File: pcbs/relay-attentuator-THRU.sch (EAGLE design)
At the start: 25 parts, among them IC1 ULN2803, IC2 MCP23S08, K1 IM23TS, K2 IM43TS, K3 IM43TS, K4 IM43TS, X1 22-23-2051

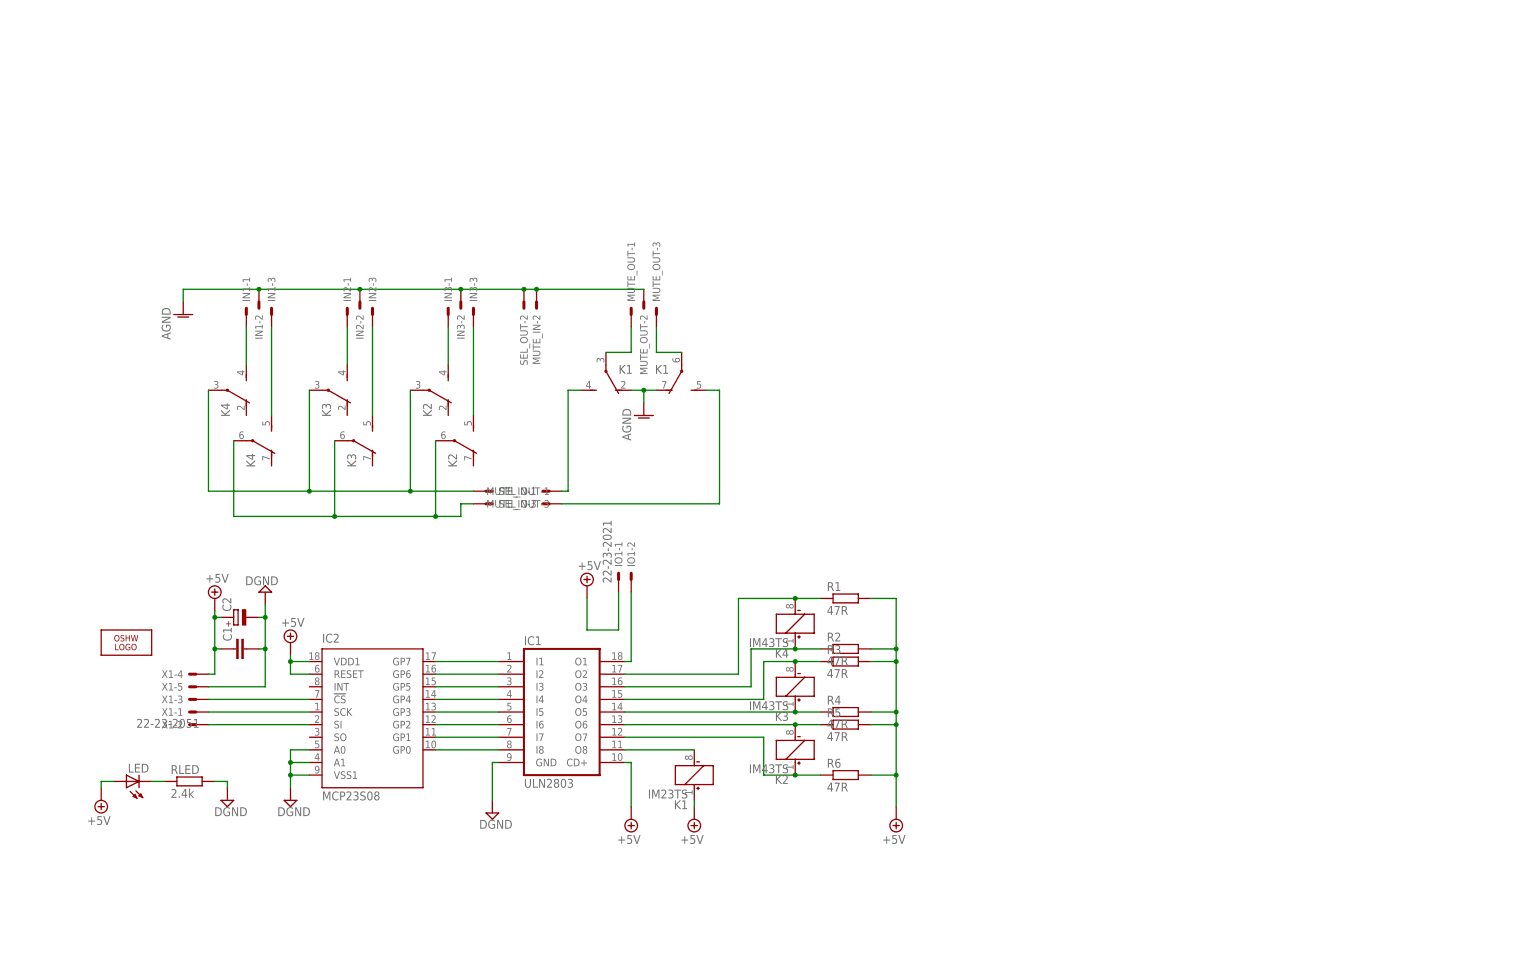
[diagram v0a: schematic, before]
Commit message: new designs
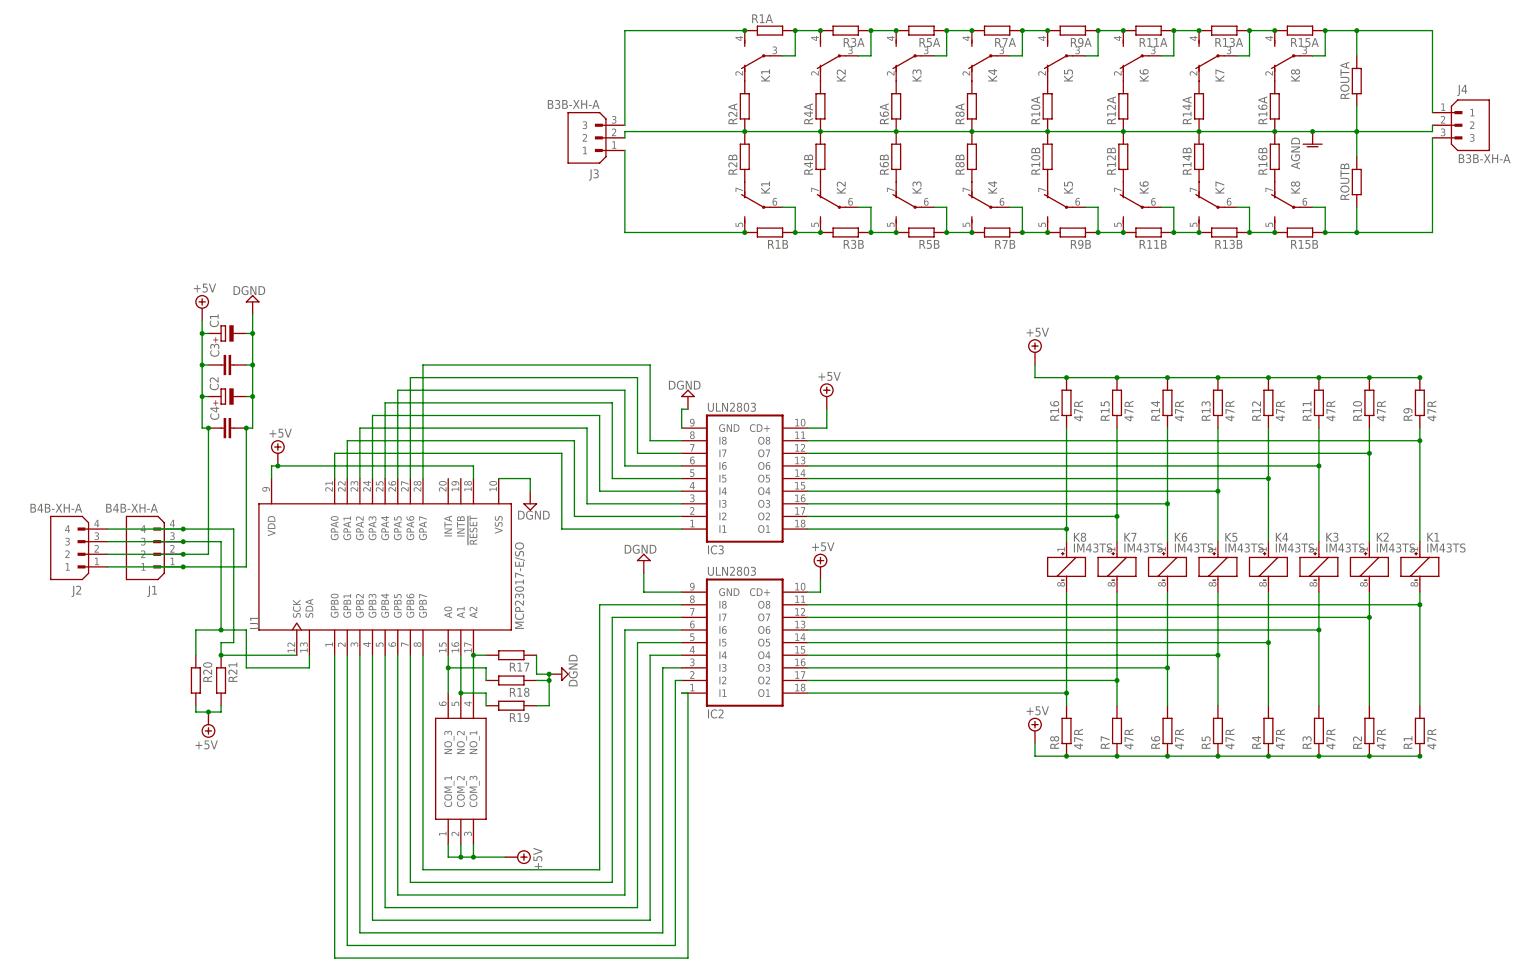
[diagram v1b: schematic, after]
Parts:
- removed IC1: ULN2803, uln-udn-mine:ULN2803ADW
- removed IN1, IN2, IN3, MUTE_IN, MUTE_OUT, SEL_OUT: 22-23-2031, con-molex:22-23-2031
- removed IO1: 22-23-2021, con-molex:22-23-2021
- removed LED: (no value), led:LEDCHIPLED_1206
- removed LOGO1: OSHW_LOGO_FILLX0200-NT, ohw-logo:OSHW_LOGO_FILLX0200-NT
- removed RLED: 2.4k, rcl:R-EU_R1206
- removed X1: 22-23-2051, con-molex:22-23-2051
- added C3, C4: (no value), rcl:C-EUC1206
- added IC3: ULN2803, uln-udn-mine:ULN2803ADW
- added J1, J2: B4B-XH-A, B4B-XH-A:B4B-XH-A
- added J3, J4: B3B-XH-A, B3B-XH-A:B3B-XH-A
- added K5, K6, K7, K8: IM43TS, relay-te:IM43TS
- added R10, R11, R12, R13, R14, R15, R16, R17, R18, R19, R20, R21, R7, R8, R9: 47R, rcl:R-EU_R1206
- added R10A, R10B, R11A, R11B, R12A, R12B, R13A, R13B, R14A, R14B, R15A, R15B, R16A, R16B, R1A, R1B, R2A, R2B, R3A, R3B, R4A, R4B, R5A, R5B, R6A, R6B, R7A, R7B, R8A, R8B, R9A, R9B, ROUTA, ROUTB: (no value), rcl:R-EU_0207/10
- added S1: 2454982-2, 2454982-2:2454982-2
- added U1: MCP23017-E/SO, MCP23017-E_SO:MCP23017-E/SO
- C1: device rcl:C-EUC1206 -> rcl:CPOL-EUE3.5-8
- C2: device rcl:CPOL-EUC -> rcl:CPOL-EUE3.5-8
- IC2: value MCP23S08 -> ULN2803; device microchip-mine:MCP23S08-E/SO -> uln-udn-mine:ULN2803ADW
- K1: value IM23TS -> IM43TS; device relay-te:IM23TS -> relay-te:IM43TS
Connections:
- removed net CS: IC2.!CS, X1-3.S
- removed net INL: K22.P, K32.P, K42.P, SEL_OUT-1.S
- removed net INR: K23.P, K33.P, K43.P, SEL_OUT-3.S
- removed net N$67: LED.C, RLED.1
- removed net OUTL: K12.S, MUTE_IN-1.S
- removed net OUTR: K13.S, MUTE_IN-3.S
- removed net SCK: IC2.SCK, X1-1.S
- removed net SI: IC2.SI, X1-2.S
- new net ATT_INR: J3.1, K13.S, R1B.2
- new net N$114: K32.P, K42.S, R5A.1, R7A.2
- new net N$115: K42.P, K52.S, R7A.1, R9A.2
- new net N$116: K52.P, K62.S, R11A.2, R9A.1
- new net N$117: K62.P, K72.S, R11A.1, R13A.2
- new net N$120: K23.P, K33.S, R3B.1, R5B.2
- new net N$121: K33.P, K43.S, R5B.1, R7B.2
- new net N$122: K43.P, K53.S, R7B.1, R9B.2
- new net N$123: K53.P, K63.S, R11B.2, R9B.1
- new net N$19: IC2.O3, K61.-, R6.2
- new net N$20: IC2.O4, K51.-, R5.2
- new net N$21: K43.O, R8B.1
- new net N$22: K53.O, R10B.1
- new net N$23: K63.O, R12B.1
- new net N$24: K73.O, R14B.1
- new net N$25: K83.O, R16B.1
- new net N$26: K22.O, R4A.2
- new net N$27: K32.O, R6A.2
- new net N$28: K42.O, R8A.2
- new net N$29: K52.O, R10A.2
- new net N$30: K62.O, R12A.2
- new net N$37: IC2.I4, U1.GPB3
- new net N$38: IC2.I3, U1.GPB2
- new net N$39: IC2.I2, U1.GPB1
- new net N$40: IC2.I1, U1.GPB0
- new net N$41: IC3.I1, U1.GPA0
- new net N$42: IC3.I2, U1.GPA1
- new net N$43: IC3.I3, U1.GPA2
- new net N$44: IC3.I4, U1.GPA3
- new net N$45: IC3.I5, U1.GPA4
- new net N$46: IC3.I6, U1.GPA5
- new net N$47: IC3.I7, U1.GPA6
- new net N$48: IC3.I8, U1.GPA7
- new net N$49: J3.3, K12.S, R1A.1
- new net N$50: K73.P, K83.S, R13B.1, R15B.2
- new net N$52: K72.P, K82.S, R13A.1, R15A.2
- new net N$55: R18.2, S1.NO_3, U1.A0
- new net N$56: R19.2, S1.NO_2, U1.A1
- new net N$57: R17.2, S1.NO_1, U1.A2
- new net N$58: J1.3, J2.3, R20.1, U1.SDA
- new net N$59: J1.4, J2.4, R21.1, U1.SCK
- new net N$61: K63.P, K73.S, R11B.1, R13B.2
- new net N$69: J4.3, K83.P, R15B.1, ROUTB.1
- new net N$71: J4.1, K82.P, R15A.1, ROUTA.2
- new net N$76: K12.P, K22.S, R1A.2, R3A.2
- new net N$80: K22.P, K32.S, R3A.1, R5A.2
- new net N$82: K13.P, K23.S, R1B.1, R3B.2
- net +5V: now also C1.+, C3.1, C4.1, IC2.CD+, IC3.CD+, J1.2, J2.2, R1.1, R10.2, R11.2, R12.2, R13.2, R14.2, R15.2, R16.2, R2.1, R20.2, R21.2, R3.1, R4.1, R5.1, R6.1, R7.1, R8.1, R9.2, S1.COM_1, S1.COM_2, S1.COM_3, U1.!RESET, U1.VDD; no longer C1.1, IC1.CD+, IC2.RESET, IC2.VDD1, IO1-1.S, K11.+, LED.A, R1.2, R2.2, R3.2, R4.2, R5.2, R6.2, X1-4.S
- net AGND: now also J3.2, J4.2, R10A.1, R10B.2, R12A.1, R12B.2, R14A.1, R14B.2, R16A.1, R16B.2, R2A.1, R2B.2, R4A.1, R4B.2, R6A.1, R6B.2, R8A.1, R8B.2, ROUTA.1, ROUTB.2; no longer IN1-2.S, IN2-2.S, IN3-2.S, K12.O, K13.O, MUTE_IN-2.S, MUTE_OUT-2.S, SEL_OUT-2.S
- net DGND: now also C1.-, C3.2, C4.2, IC2.GND, IC3.GND, J1.1, J2.1, R17.1, R18.1, R19.1, U1.VSS; no longer C1.2, IC1.GND, IC2.A0, IC2.A1, IC2.VSS1, RLED.2, X1-5.S
- net N$1: now also IC3.O1, K81.+, R16.1; no longer IC1.I1, IC2.GP7
- net N$10: now also IC3.O2, K71.+, R15.1; no longer IC1.O5, K31.+, R4.1
- net N$11: now also IC3.O3, K61.+, R14.1; no longer IC1.O6, K21.-, R5.1
- net N$12: now also IC3.O4, K51.+, R13.1; no longer IC1.O7, K21.+, R6.1
- net N$13: now also IC3.O5, K41.+, R12.1; no longer IC1.O4, K31.-, R3.1
- net N$14: now also IC3.O6, K31.+, R11.1; no longer IC1.O8, K11.-
- net N$15: now also IC3.O7, K21.+, R10.1; no longer IC1.O2, K41.-, R1.1
- net N$16: now also IC3.O8, K11.+, R9.1; no longer IC1.O1, IO1-2.S
- net N$17: now also K33.O, R6B.1; no longer K13.P, MUTE_OUT-3.S
- net N$18: now also IC2.O7, K21.-, R2.2; no longer K12.P, MUTE_OUT-1.S
- net N$2: now also IC2.O8, K11.-, R1.2; no longer IC1.I2, IC2.GP6
- net N$3: now also IC2.O2, K71.-, R7.2; no longer IC1.I3, IC2.GP5
- net N$31: now also K72.O, R14A.2; no longer IN1-1.S, K42.S
- net N$32: now also K82.O, R16A.2; no longer IN1-3.S, K43.S
- net N$33: now also IC2.I8, U1.GPB7; no longer IN2-1.S, K32.S
- net N$34: now also IC2.I7, U1.GPB6; no longer IN2-3.S, K33.S
- net N$35: now also IC2.I6, U1.GPB5; no longer IN3-1.S, K22.S
- net N$36: now also IC2.I5, U1.GPB4; no longer IN3-3.S, K23.S
- net N$4: now also IC2.O6, K31.-, R3.2; no longer IC1.I5, IC2.GP3
- net N$5: now also IC2.O5, K41.-, R4.2; no longer IC1.I6, IC2.GP2
- net N$6: now also K23.O, R4B.1; no longer IC1.I7, IC2.GP1
- net N$7: now also K13.O, R2B.1; no longer IC1.I4, IC2.GP4
- net N$8: now also K12.O, R2A.2; no longer IC1.I8, IC2.GP0
- net N$9: now also IC2.O1, K81.-, R8.2; no longer IC1.O3, K41.+, R2.1
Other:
- moved on the sheet: C2, IC2, K1, K2, K3, K4, R1, R2, R3, R4, R5, R6
